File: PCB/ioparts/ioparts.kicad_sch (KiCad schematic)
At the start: 10 parts, among them J1 USB_B_Micro, J2 USB_C_Receptacle_USB2.0, J3 Conn_01x04, J4 Conn_01x04, J5 AudioJack4, J6 AudioJack4, J7 Conn_01x04, J8 Conn_01x04

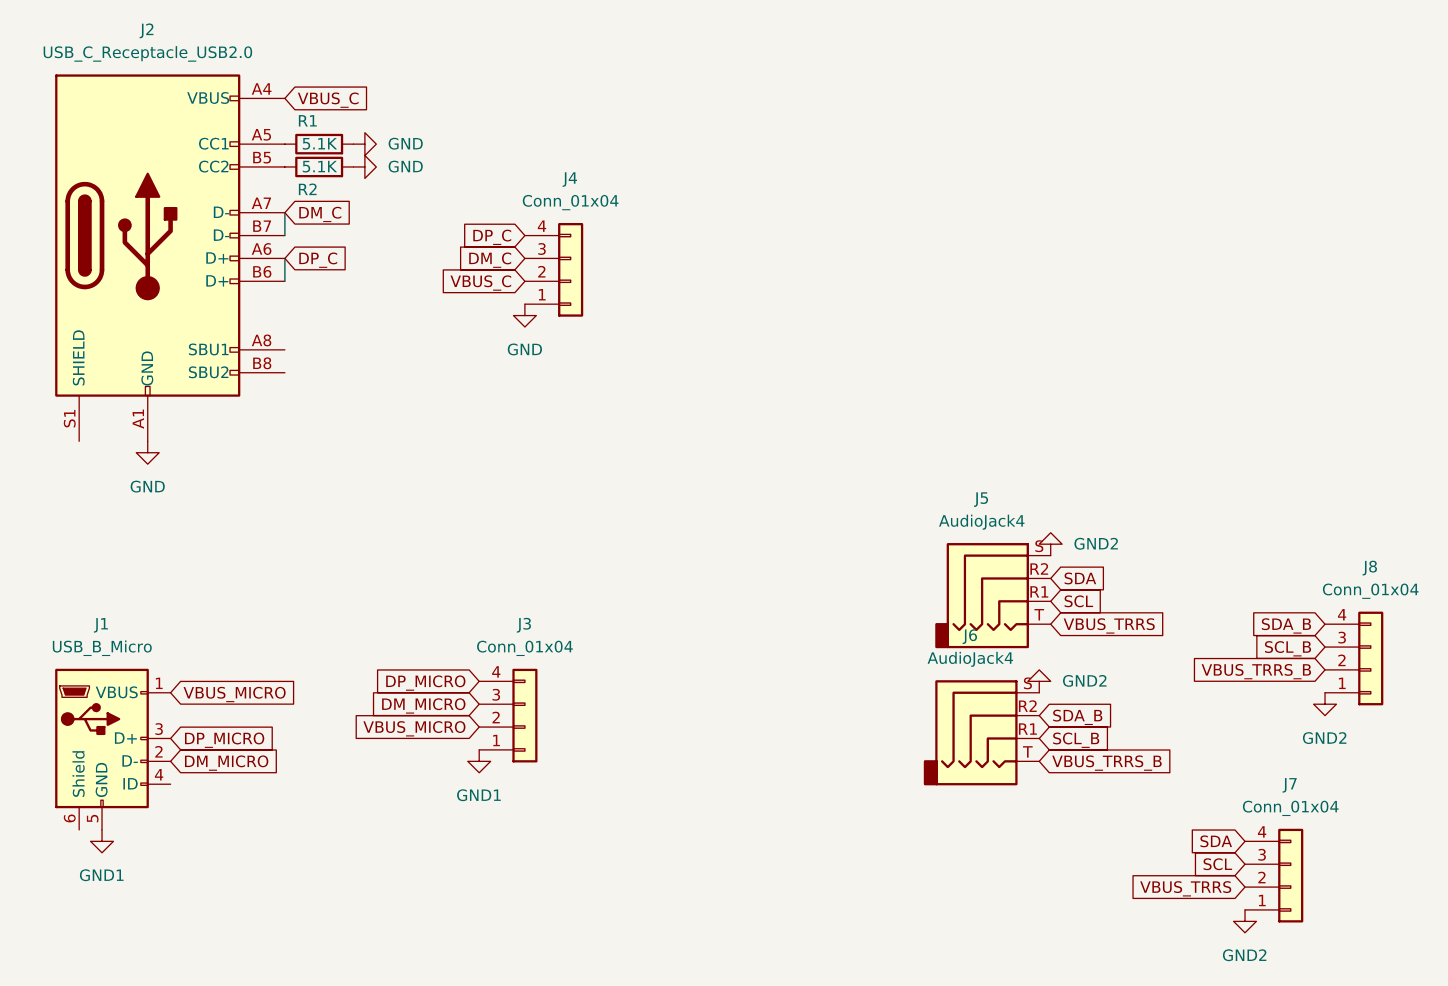
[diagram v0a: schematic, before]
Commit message: temp
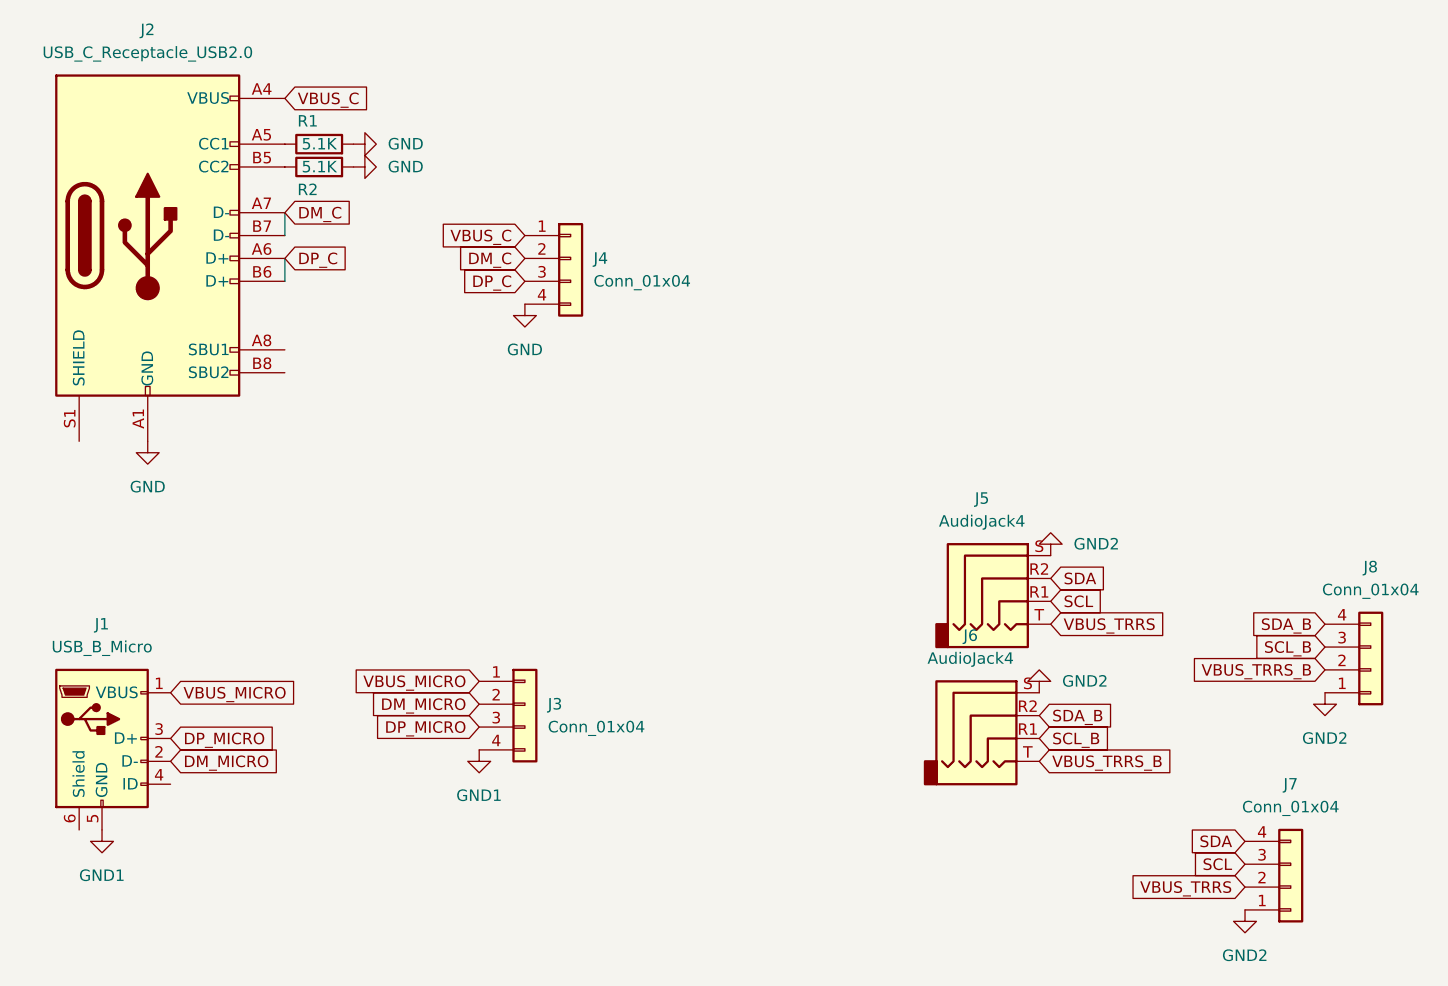
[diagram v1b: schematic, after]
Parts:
- J2: footprint ioparts:KH-TYPE-C-L10-14P -> Connector_USB:USB_C_Receptacle_HRO_TYPE-C-31-M-12
- J3: footprint Connector_JST:JST_SH_SM04B-SRSS-TB_1x04-1MP_P1.00mm_Horizontal -> Connector_JST:JST_PH_S4B-PH-K_1x04_P2.00mm_Horizontal
- J4: footprint Connector_JST:JST_SH_BM04B-SRSS-TB_1x04-1MP_P1.00mm_Vertical -> Connector_JST:JST_PH_S4B-PH-K_1x04_P2.00mm_Horizontal
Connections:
- net DM_C: now also J4.2 (Pin_2); no longer J4.3 (Pin_3)
- net DM_MICRO: now also J3.2 (Pin_2); no longer J3.3 (Pin_3)
- net DP_C: now also J4.3 (Pin_3); no longer J4.4 (Pin_4)
- net DP_MICRO: now also J3.3 (Pin_3); no longer J3.4 (Pin_4)
- net GND: now also J4.4 (Pin_4); no longer J4.1 (Pin_1)
- net GND1: now also J3.4 (Pin_4); no longer J3.1 (Pin_1)
- net VBUS_C: now also J4.1 (Pin_1); no longer J4.2 (Pin_2)
- net VBUS_MICRO: now also J3.1 (Pin_1); no longer J3.2 (Pin_2)
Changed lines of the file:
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@@
-    )
-  )
-  (global_label "VBUS_C" (shape input) (at 118.11 64.77 180) (fields_autoplaced)
-    (effects (font (size 1.27 1.27)) (justify right))
-    (property "Intersheet References" "${INTERSHEET_REFS}" (id 0) (at 108.5607 64.6906 0)
-      (effects (font (size 1.27 1.27)) (justify right) hide)
     )
   )
@@
     )
   )
+  (global_label "DP_MICRO" (shape input) (at 113.03 114.3 180) (fields_autoplaced)
+    (effects (font (size 1.27 1.27)) (justify right))
+    (property "Intersheet References" "${INTERSHEET_REFS}" (id 0) (at 101.1826 114.2206 0)
+      (effects (font (size 1.27 1.27)) (justify right) hide)
+    )
+  )
   (global_label "VBUS_TRRS_B" (shape input) (at 207.01 107.95 180) (fields_autoplaced)
     (effects (font (size 1.27 1.27)) (justify right))
@@
     )
   )
-  (global_label "DP_MICRO" (shape input) (at 113.03 109.22 180) (fields_autoplaced)
-    (effects (font (size 1.27 1.27)) (justify right))
-    (property "Intersheet References" "${INTERSHEET_REFS}" (id 0) (at 101.1826 109.1406 0)
-      (effects (font (size 1.27 1.27)) (justify right) hide)
-    )
-  )
-  (global_label "DP_C" (shape input) (at 118.11 59.69 180) (fields_autoplaced)
-    (effects (font (size 1.27 1.27)) (justify right))
-    (property "Intersheet References" "${INTERSHEET_REFS}" (id 0) (at 110.9193 59.6106 0)
+  (global_label "DM_MICRO" (shape input) (at 113.03 111.76 180) (fields_autoplaced)
+    (effects (font (size 1.27 1.27)) (justify right))
+    (property "Intersheet References" "${INTERSHEET_REFS}" (id 0) (at 101.0012 111.6806 0)
+      (effects (font (size 1.27 1.27)) (justify right) hide)
+    )
+  )
+  (global_label "DP_C" (shape input) (at 118.11 64.77 180) (fields_autoplaced)
+    (effects (font (size 1.27 1.27)) (justify right))
+    (property "Intersheet References" "${INTERSHEET_REFS}" (id 0) (at 110.9193 64.6906 0)
       (effects (font (size 1.27 1.27)) (justify right) hide)
     )
@@
     )
   )
+  (global_label "VBUS_MICRO" (shape input) (at 113.03 109.22 180) (fields_autoplaced)
+    (effects (font (size 1.27 1.27)) (justify right))
+    (property "Intersheet References" "${INTERSHEET_REFS}" (id 0) (at 98.824 109.2994 0)
+      (effects (font (size 1.27 1.27)) (justify right) hide)
+    )
+  )
   (global_label "SDA" (shape input) (at 198.12 127 180) (fields_autoplaced)
     (effects (font (size 1.27 1.27)) (justify right))
@@
     )
   )
-  (global_label "DM_MICRO" (shape input) (at 113.03 111.76 180) (fields_autoplaced)
-    (effects (font (size 1.27 1.27)) (justify right))
-    (property "Intersheet References" "${INTERSHEET_REFS}" (id 0) (at 101.0012 111.6806 0)
-      (effects (font (size 1.27 1.27)) (justify right) hide)
-    )
-  )
-  (global_label "VBUS_MICRO" (shape input) (at 113.03 114.3 180) (fields_autoplaced)
-    (effects (font (size 1.27 1.27)) (justify right))
-    (property "Intersheet References" "${INTERSHEET_REFS}" (id 0) (at 98.824 114.3794 0)
-      (effects (font (size 1.27 1.27)) (justify right) hide)
-    )
-  )
   (global_label "DM_C" (shape input) (at 118.11 62.23 180) (fields_autoplaced)
     (effects (font (size 1.27 1.27)) (justify right))
@@
     (property "Intersheet References" "${INTERSHEET_REFS}" (id 0) (at 182.4507 100.2506 0)
       (effects (font (size 1.27 1.27)) (justify left) hide)
+    )
+  )
+  (global_label "VBUS_C" (shape input) (at 118.11 59.69 180) (fields_autoplaced)
+    (effects (font (size 1.27 1.27)) (justify right))
+    (property "Intersheet References" "${INTERSHEET_REFS}" (id 0) (at 108.5607 59.6106 0)
+      (effects (font (size 1.27 1.27)) (justify right) hide)
     )
   )
@@
     (property "Reference" "J2" (id 0) (at 76.2 36.83 0))
     (property "Value" "USB_C_Receptacle_USB2.0" (id 1) (at 76.2 39.37 0))
-    (property "Footprint" "ioparts:KH-TYPE-C-L10-14P" (id 2) (at 80.01 59.69 0)
+    (property "Footprint" "Connector_USB:USB_C_Receptacle_HRO_TYPE-C-31-M-12" (id 2) (at 80.01 59.69 0)
       (effects (font (size 1.27 1.27)) hide)
     )
@@
     (pin "6")
   )
+  (symbol (lib_id "Connector_Generic:Conn_01x04") (at 123.19 62.23 0) (unit 1)
+    (in_bom yes) (on_board yes) (fields_autoplaced)
+    (property "Reference" "J4" (id 0) (at 125.73 62.2299 0)
+      (effects (font (size 1.27 1.27)) (justify left))
+    )
+    (property "Value" "Conn_01x04" (id 1) (at 125.73 64.7699 0)
+      (effects (font (size 1.27 1.27)) (justify left))
+    )
+    (property "Footprint" "Connector_JST:JST_PH_S4B-PH-K_1x04_P2.00mm_Horizontal" (id 2) (at 123.19 62.23 0)
+      (effects (font (size 1.27 1.27)) hide)
+    )
+    (property "Datasheet" "~" (id 3) (at 123.19 62.23 0)
+      (effects (font (size 1.27 1.27)) hide)
+    )
+    (pin "1")
+    (pin "2")
+    (pin "3")
+    (pin "4")
+  )
   (symbol (lib_id "power:GND1") (at 71.12 125.73 0) (unit 1)
     (in_bom yes) (on_board yes) (fields_autoplaced)
@@
     (pin "T")
   )
-  (symbol (lib_id "Connector_Generic:Conn_01x04") (at 123.19 64.77 0) (mirror x) (unit 1)
-    (in_bom yes) (on_board yes) (fields_autoplaced)
-    (property "Reference" "J4" (id 0) (at 123.19 53.34 0))
-    (property "Value" "Conn_01x04" (id 1) (at 123.19 55.88 0))
-    (property "Footprint" "Connector_JST:JST_SH_BM04B-SRSS-TB_1x04-1MP_P1.00mm_Vertical" (id 2) (at 123.19 64.77 0)
-      (effects (font (size 1.27 1.27)) hide)
-    )
-    (property "Datasheet" "~" (id 3) (at 123.19 64.77 0)
+  (symbol (lib_id "Connector_Generic:Conn_01x04") (at 118.11 111.76 0) (unit 1)
+    (in_bom yes) (on_board yes) (fields_autoplaced)
+    (property "Reference" "J3" (id 0) (at 120.65 111.7599 0)
+      (effects (font (size 1.27 1.27)) (justify left))
+    )
+    (property "Value" "Conn_01x04" (id 1) (at 120.65 114.2999 0)
+      (effects (font (size 1.27 1.27)) (justify left))
+    )
+    (property "Footprint" "Connector_JST:JST_PH_S4B-PH-K_1x04_P2.00mm_Horizontal" (id 2) (at 118.11 111.76 0)
+      (effects (font (size 1.27 1.27)) hide)
+    )
+    (property "Datasheet" "~" (id 3) (at 118.11 111.76 0)
       (effects (font (size 1.27 1.27)) hide)
     )
@@
     (pin "T")
   )
-  (symbol (lib_id "Connector_Generic:Conn_01x04") (at 118.11 114.3 0) (mirror x) (unit 1)
-    (in_bom yes) (on_board yes)
-    (property "Reference" "J3" (id 0) (at 118.11 102.87 0))
-    (property "Value" "Conn_01x04" (id 1) (at 118.11 105.41 0))
-    (property "Footprint" "Connector_JST:JST_SH_SM04B-SRSS-TB_1x04-1MP_P1.00mm_Horizontal" (id 2) (at 118.11 114.3 0)
-      (effects (font (size 1.27 1.27)) hide)
-    )
-    (property "Datasheet" "~" (id 3) (at 118.11 114.3 0)
-      (effects (font (size 1.27 1.27)) hide)
-    )
-    (pin "1")
-    (pin "2")
-    (pin "3")
-    (pin "4")
-  )
   (symbol (lib_id "power:GND2") (at 176.53 95.25 180) (unit 1)
     (in_bom yes) (on_board yes) (fields_autoplaced)
@@
     )
     (path "/2f4f8505-9ff9-401a-9e46-f206a08f2e88"
-      (reference "J2") (unit 1) (value "USB_C_Receptacle_USB2.0") (footprint "ioparts:KH-TYPE-C-L10-14P")
-    )
-    (path "/da983080-025b-4fc0-b7b9-25e30f08b91c"
-      (reference "J3") (unit 1) (value "Conn_01x04") (footprint "Connector_JST:JST_SH_SM04B-SRSS-TB_1x04-1MP_P1.00mm_Horizontal")
-    )
-    (path "/b8a83813-4e90-4ac5-920d-f6cd36104aae"
-      (reference "J4") (unit 1) (value "Conn_01x04") (footprint "Connector_JST:JST_SH_BM04B-SRSS-TB_1x04-1MP_P1.00mm_Vertical")
+      (reference "J2") (unit 1) (value "USB_C_Receptacle_USB2.0") (footprint "Connector_USB:USB_C_Receptacle_HRO_TYPE-C-31-M-12")
+    )
+    (path "/b9a92b39-e387-41bf-9641-9883e116b75e"
+      (reference "J3") (unit 1) (value "Conn_01x04") (footprint "Connector_JST:JST_PH_S4B-PH-K_1x04_P2.00mm_Horizontal")
+    )
+    (path "/830ece5e-48d8-41a3-a25c-ad05159ec093"
+      (reference "J4") (unit 1) (value "Conn_01x04") (footprint "Connector_JST:JST_PH_S4B-PH-K_1x04_P2.00mm_Horizontal")
     )
     (path "/b08805d0-ca9c-4850-9c1f-d4fb4e24076f"
